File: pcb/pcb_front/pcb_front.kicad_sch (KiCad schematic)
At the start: 24 parts, among them J1 MicroLab, J2 LED_BREAKOUT, J3 GAS_BREAKOUT, U1 TBD62783A

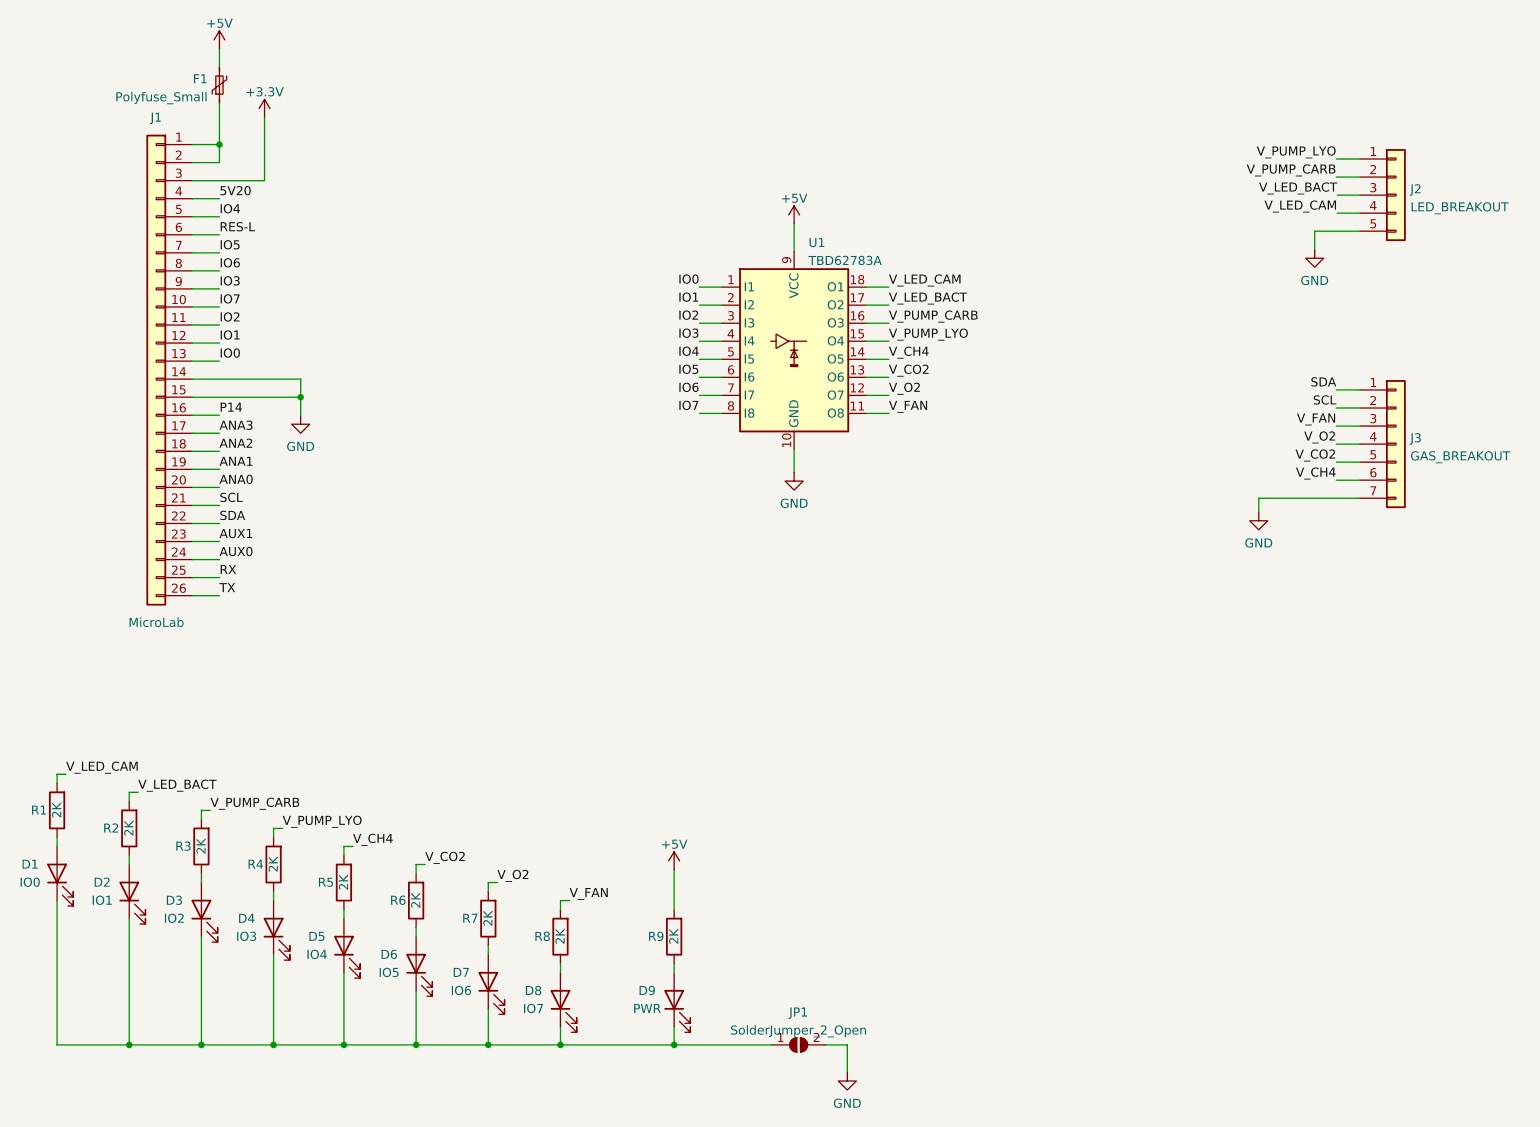
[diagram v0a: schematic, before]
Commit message: front pcb rev 2
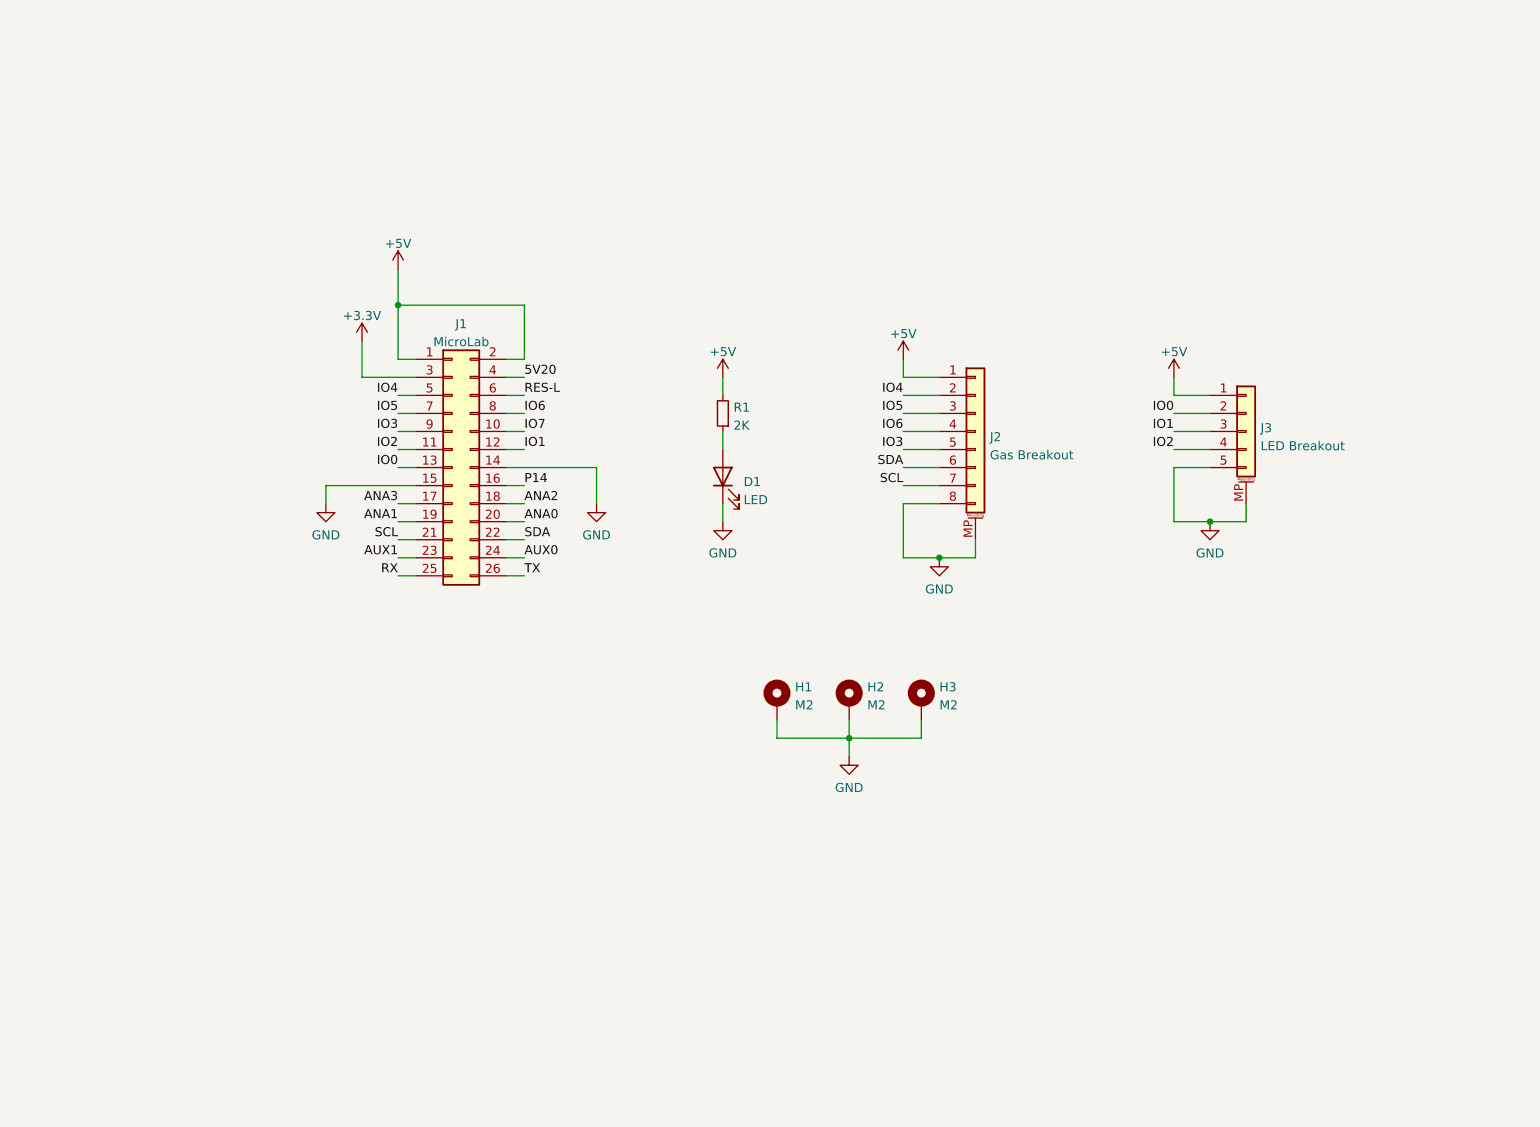
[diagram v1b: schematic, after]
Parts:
- removed D2: IO1, LED_SMD:LED_0603_1608Metric, symbol Device:LED
- removed D3: IO2, LED_SMD:LED_0603_1608Metric, symbol Device:LED
- removed D4: IO3, LED_SMD:LED_0603_1608Metric, symbol Device:LED
- removed D5: IO4, LED_SMD:LED_0603_1608Metric, symbol Device:LED
- removed D6: IO5, LED_SMD:LED_0603_1608Metric, symbol Device:LED
- removed D7: IO6, LED_SMD:LED_0603_1608Metric, symbol Device:LED
- removed D8: IO7, LED_SMD:LED_0603_1608Metric, symbol Device:LED
- removed D9: PWR, LED_SMD:LED_0603_1608Metric, symbol Device:LED
- removed F1: Polyfuse_Small, Fuse:Fuse_0603_1608Metric, symbol Device:Polyfuse_Small
- removed J1: MicroLab, Connector_PinSocket_2.00mm:PinSocket_2x13_P2.00mm_Horizontal, symbol Connector_Generic:Conn_01x26
- removed J2: LED_BREAKOUT, Connector_JST:JST_SH_SM05B-SRSS-TB_1x05-1MP_P1.00mm_Horizontal, symbol Connector_Generic:Conn_01x05
- removed J3: GAS_BREAKOUT, Connector_JST:JST_SH_SM07B-SRSS-TB_1x07-1MP_P1.00mm_Horizontal, symbol Connector_Generic:Conn_01x07
- removed JP1: SolderJumper_2_Open, Jumper:SolderJumper-2_P1.3mm_Open_TrianglePad1.0x1.5mm, symbol Jumper:SolderJumper_2_Open
- removed R1, R2, R3, R4, R5, R6, R7, R8, R9: 2K, Resistor_SMD:R_0603_1608Metric, symbol Device:R
- removed U1: TBD62783A, Package_DIP:DIP-18_W7.62mm_Socket, symbol Transistor_Array:TBD62783A
- added H1, H2, H3: M2, MountingHole:MountingHole_2.2mm_M2_DIN965_Pad, symbol Mechanical:MountingHole_Pad
- added J1: MicroLab, Connector_PinHeader_2.00mm:PinHeader_2x13_P2.00mm_Vertical, symbol Connector_Generic:Conn_02x13_Odd_Even
- added J2: Gas Breakout, Connector_JST:JST_SH_BM08B-SRSS-TB_1x08-1MP_P1.00mm_Vertical, symbol Connector_Generic_MountingPin:Conn_01x08_MountingPin
- added J3: LED Breakout, Connector_JST:JST_SH_BM05B-SRSS-TB_1x05-1MP_P1.00mm_Vertical, symbol Connector_Generic_MountingPin:Conn_01x05_MountingPin
- added R1: 2K, Resistor_SMD:R_0402_1005Metric_Pad0.72x0.64mm_HandSolder, symbol Device:R_Small
- D1: value IO0 -> LED; footprint LED_SMD:LED_0603_1608Metric -> LED_SMD:LED_0402_1005Metric_Pad0.77x0.64mm_HandSolder
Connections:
- net +3.3V: now also J1.3 (Pin_3)
- net +5V: now also J1.1 (Pin_1), J1.2 (Pin_2), J2.1 (Pin_1), J3.1 (Pin_1), R1.2
- net 5V20: now also J1.4 (Pin_4)
- net ANA0: now also J1.20 (Pin_20)
- net ANA1: now also J1.19 (Pin_19)
- net ANA2: now also J1.18 (Pin_18)
- net ANA3: now also J1.17 (Pin_17)
- net AUX0: now also J1.24 (Pin_24)
- net AUX1: now also J1.23 (Pin_23)
- net GND: now also D1.1 (K), H1.1, H2.1, H3.1, J1.14 (Pin_14), J1.15 (Pin_15), J2.8 (Pin_8), J2.MP (MountPin), J3.5 (Pin_5), J3.MP (MountPin)
- net IO0: now also J1.13 (Pin_13), J3.2 (Pin_2)
- net IO1: now also J1.12 (Pin_12), J3.3 (Pin_3)
- net IO2: now also J1.11 (Pin_11), J3.4 (Pin_4)
- net IO3: now also J1.9 (Pin_9), J2.5 (Pin_5)
- net IO4: now also J1.5 (Pin_5), J2.2 (Pin_2)
- net IO5: now also J1.7 (Pin_7), J2.3 (Pin_3)
- net IO6: now also J1.8 (Pin_8), J2.4 (Pin_4)
- net IO7: now also J1.10 (Pin_10)
- net P14: now also J1.16 (Pin_16)
- net RES-L: now also J1.6 (Pin_6)
- net RX: now also J1.25 (Pin_25)
- net SCL: now also J1.21 (Pin_21), J2.7 (Pin_7)
- net SDA: now also J1.22 (Pin_22), J2.6 (Pin_6)
- net TX: now also J1.26 (Pin_26)
- net at D1.2 (A): now also R1.1
